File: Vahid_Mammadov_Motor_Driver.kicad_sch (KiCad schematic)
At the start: 31 parts, among them J1 M1, J10 Power, J11 VCC, J12 ANALOGUE, J13 Conn_01x06_Pin, J14 Power, J15 VCC, J16 Conn_01x08_Socket, J17 Conn_01x06_Socket, J2 M2, J3 PW1, J4 PW2, J5 M3, J6 M4, J7 5V, J8 GND, J9 Power, SW1 SW_Push, U1 L293D, U2 L293D, U3 74HC595

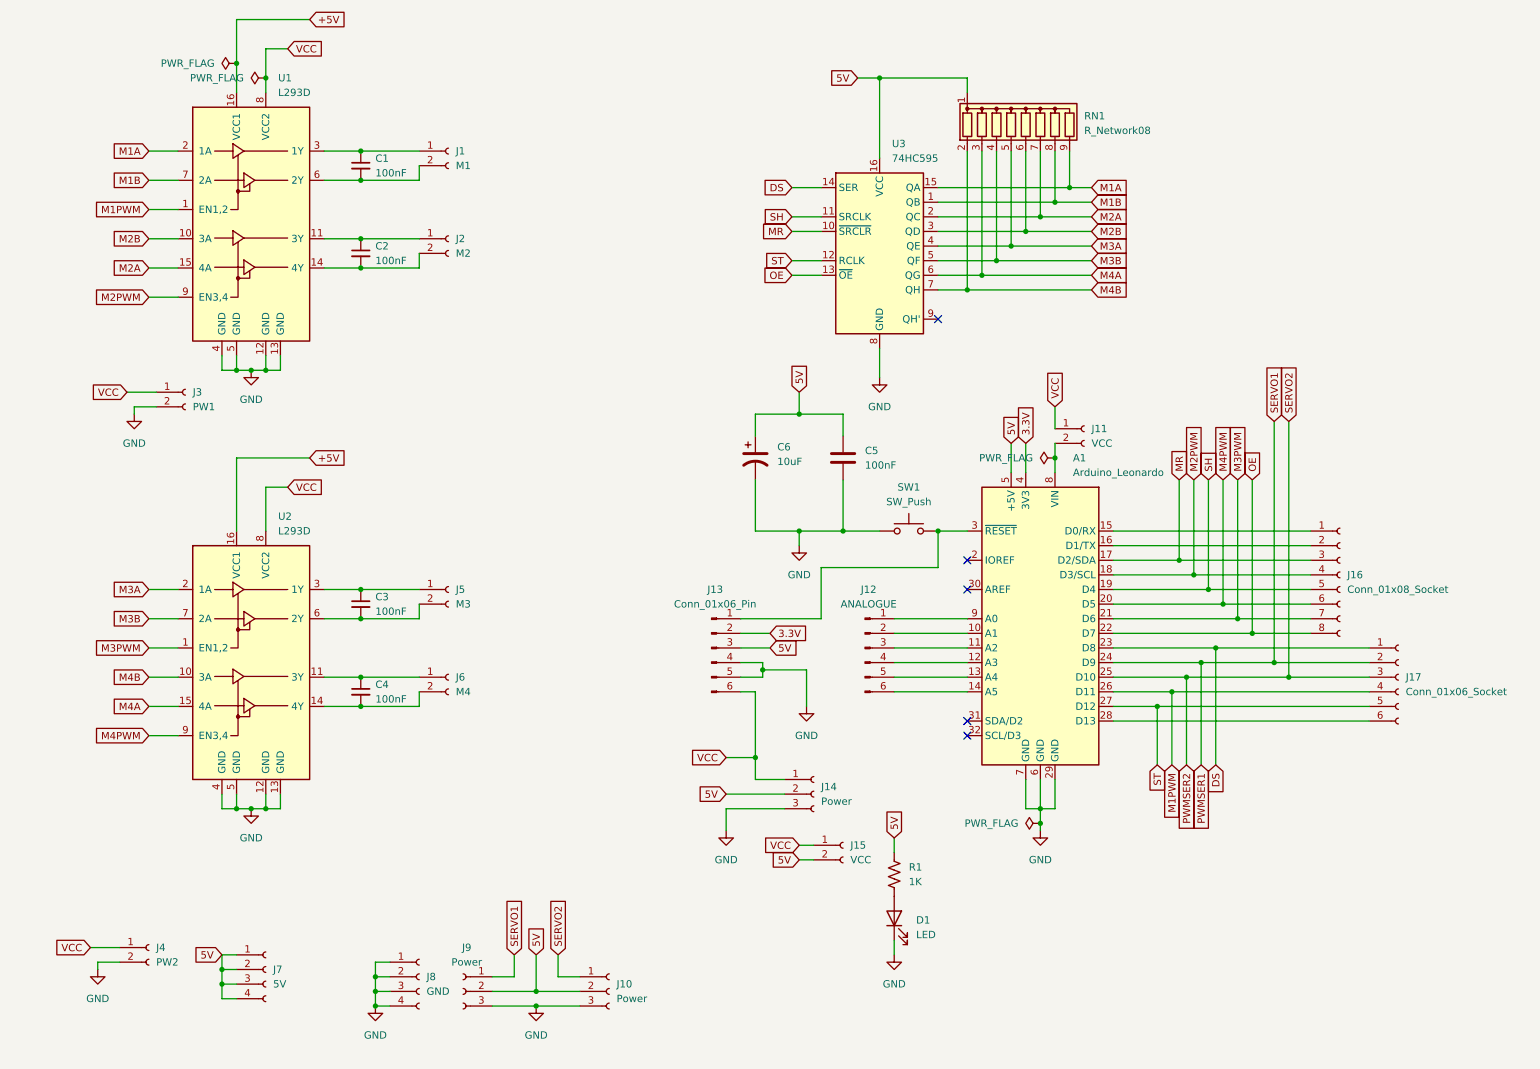
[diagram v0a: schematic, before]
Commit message: Project
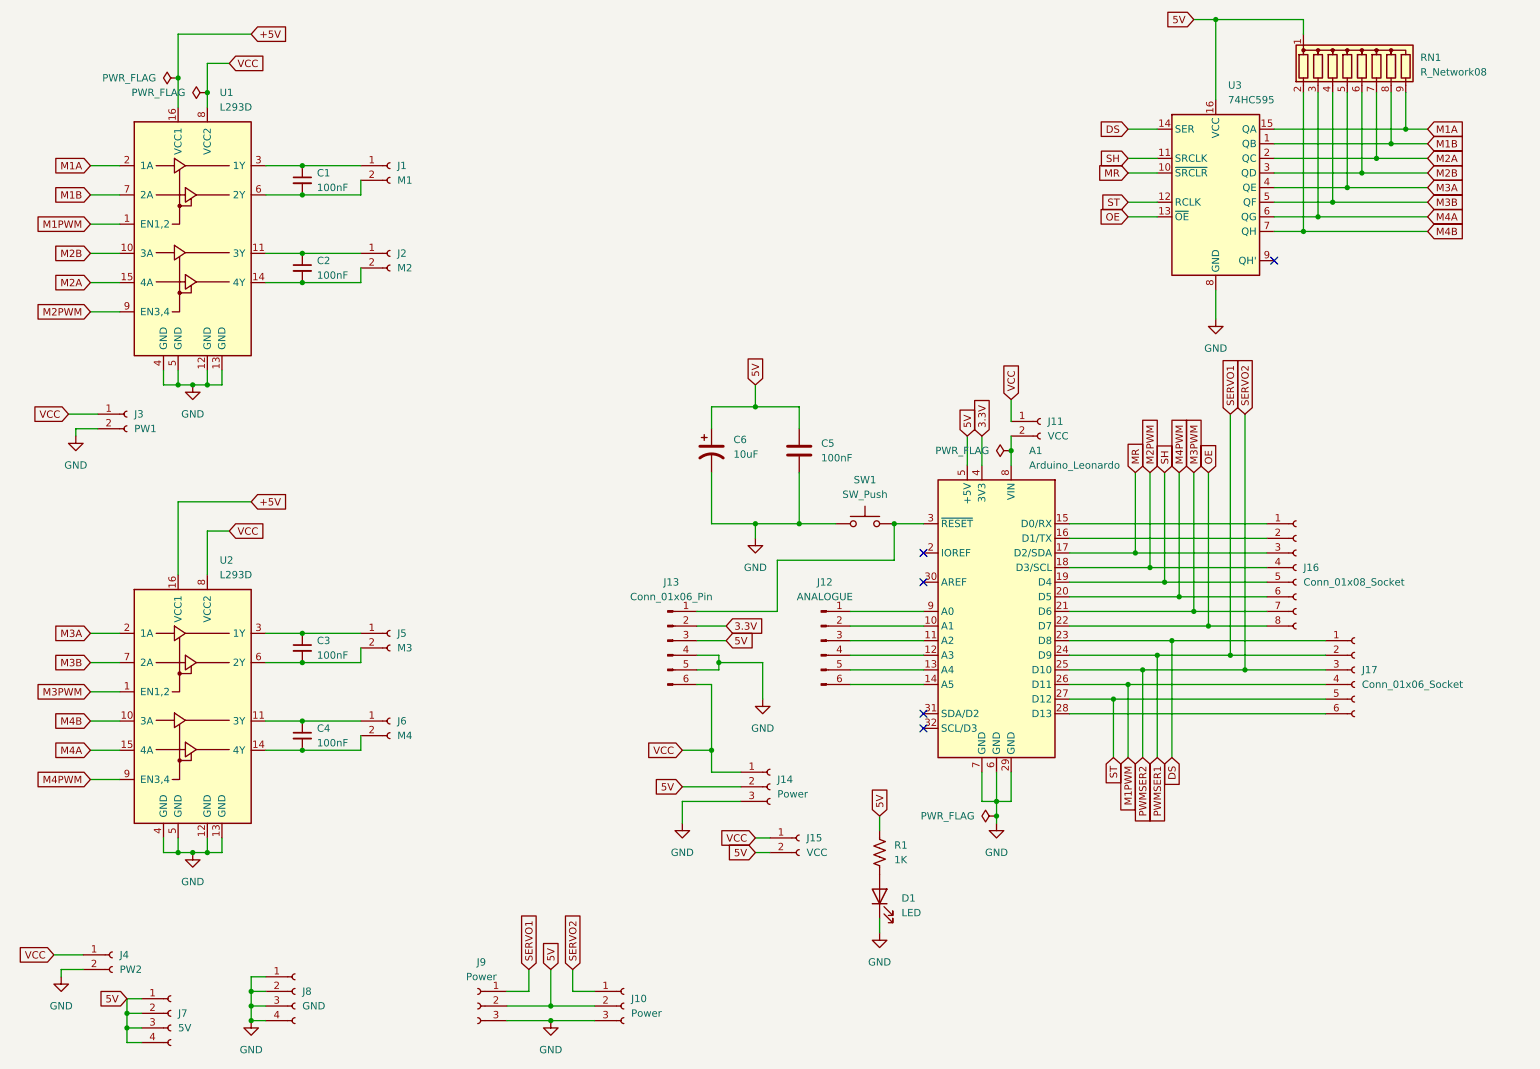
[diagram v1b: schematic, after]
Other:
- company: (none) -> bhos pae23
- title: (none) -> Motor driver - ravan
- moved on the sheet: A1, C1, C2, C3, C4, C5, C6, D1, J1, J10, J11, J12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
